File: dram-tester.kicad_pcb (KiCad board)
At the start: 2 copper layers, 53.3 x 52.1 mm, 9 parts, among them J1 Zif Socket, SW1 Reset

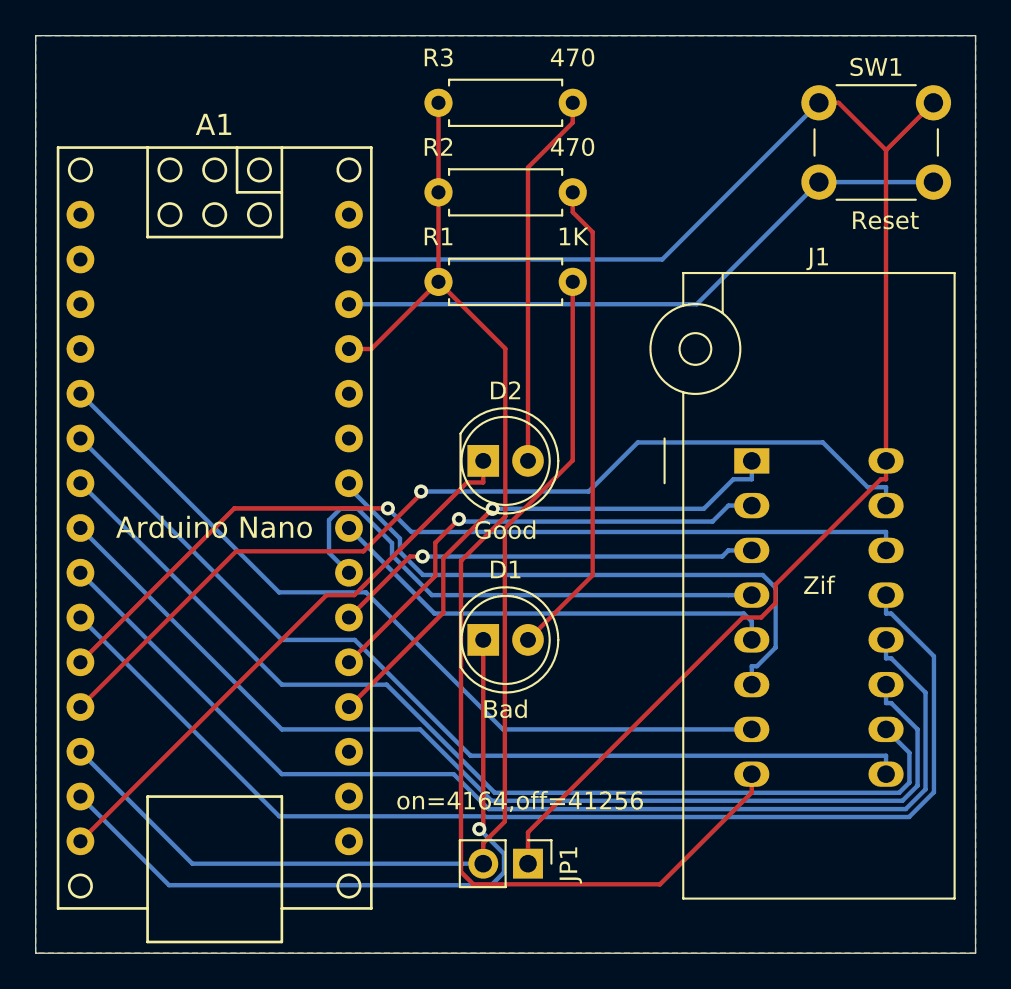
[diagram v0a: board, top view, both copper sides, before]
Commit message: cleaned up pcb
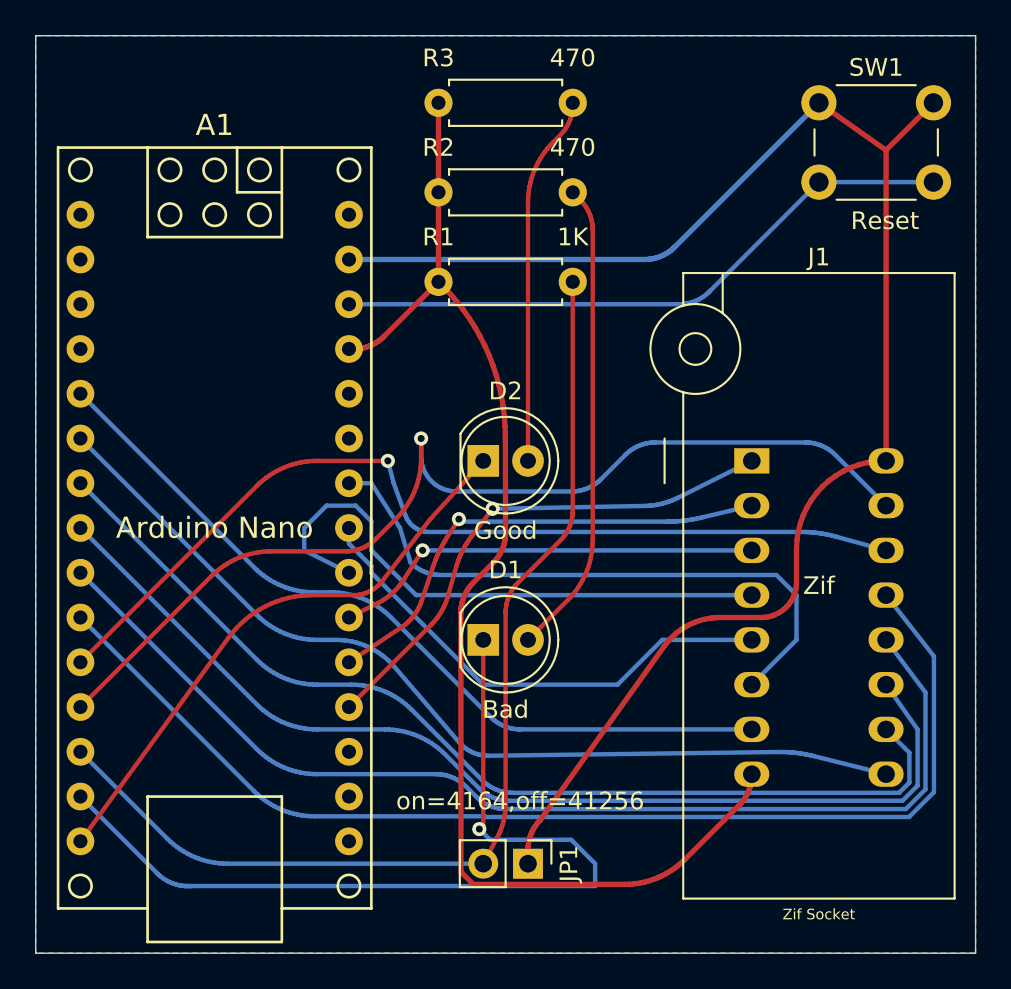
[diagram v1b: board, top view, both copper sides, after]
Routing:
- net Net-(A1-Pad14): track 40.3 -> 51.2 mm
- net Net-(A1-Pad12): track 54.1 -> 57.8 mm
- net Net-(A1-Pad22): track 30.2 -> 33.2 mm
- net Net-(A1-Pad23): track 26.1 -> 28.3 mm
- net Net-(A1-Pad11): track 50.9 -> 53.0 mm
- net Net-(A1-Pad19): track 31.1 -> 29.4 mm
- net Net-(A1-Pad24): track 33.5 -> 35.0 mm
- net Net-(A1-Pad29): track 88.8 -> 90.1 mm
- net Net-(A1-Pad6): track 54.2 -> 53.0 mm
- net Net-(A1-Pad27): track 72.9 -> 71.8 mm
- net Net-(A1-Pad8): track 60.9 -> 60.1 mm
- net Net-(A1-Pad9): track 63.6 -> 62.8 mm
- net Net-(A1-Pad13): track 60.6 -> 59.9 mm
- net Net-(A1-Pad10): track 66.2 -> 65.6 mm
- net Net-(A1-Pad7): track 58.1 -> 57.6 mm
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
